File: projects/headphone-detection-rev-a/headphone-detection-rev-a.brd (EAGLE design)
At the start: 22 x 23 mm, 9 parts, among them J1 T1M-5POS, U1 VCNL4010

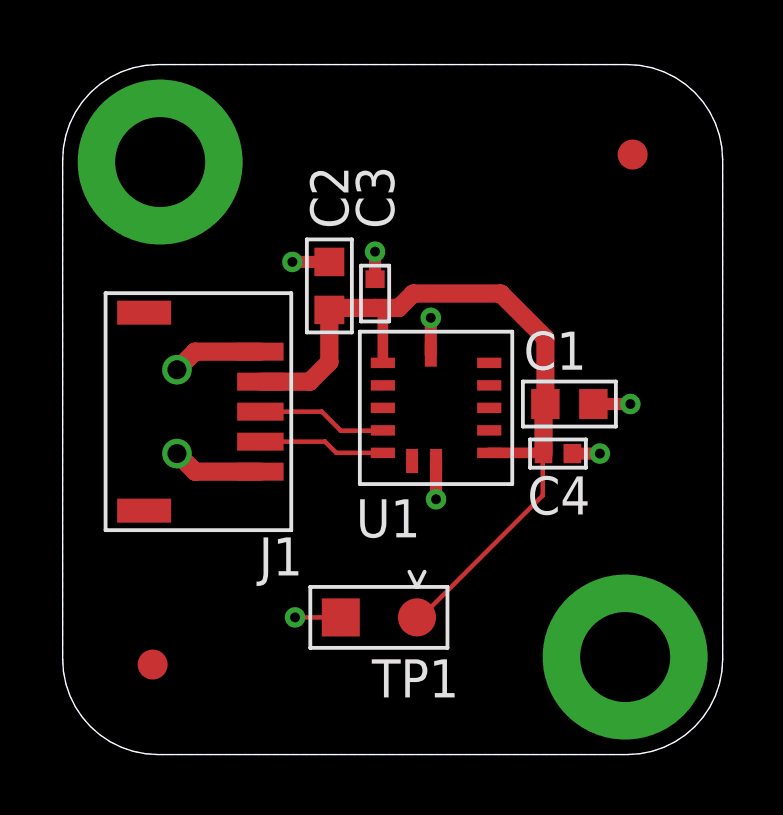
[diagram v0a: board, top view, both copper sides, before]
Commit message: Big updates to the headphone detection daughterboard.
In no particular order:

- we're now using the VL6180X (micro LIDAR, basically)
- which needs 2V8 so we have an on-board regulator
- which means we need to interface with 3V3 I2C logic so we
- added level translation FETs for each I2C line
- added test points for the two supply rails
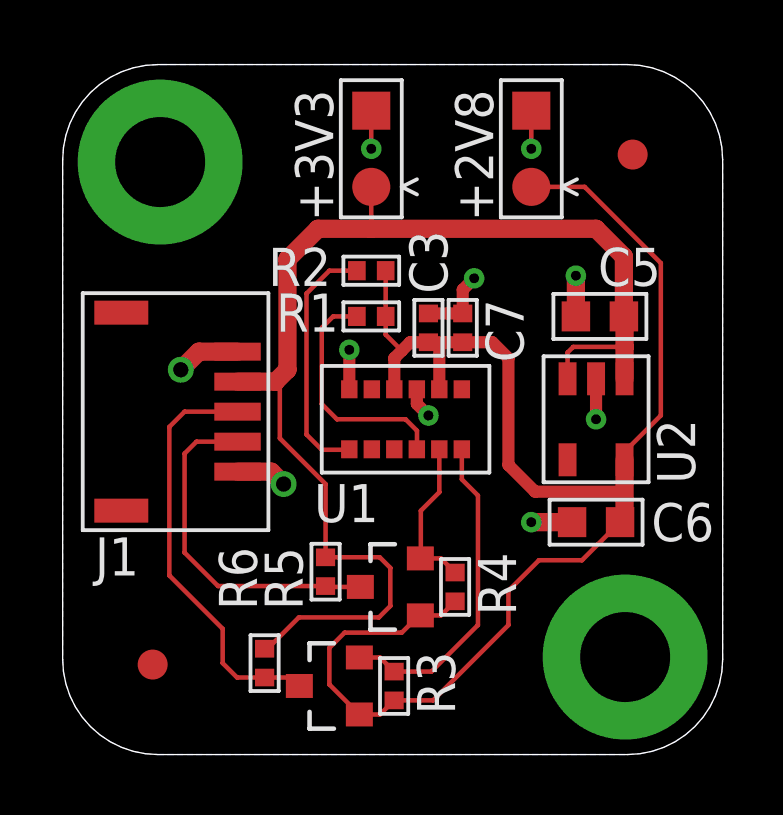
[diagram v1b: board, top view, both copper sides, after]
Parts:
- removed C1, C2: 10uF, passives:C0603
- removed C4: 1uF, passives:C0402
- added C5, C6: 10uF, passives:C0603
- added C7: 4.7uF, passives:C0402
- added R1, R2: 47K, passives:R0402
- added R3, R4, R5, R6: 10K, passives:R0402
- added TP2: TESTPOINT-WITH-GND, test:TESTPOINT-1.5-WITH-GND
- added U2: LP5907MFX-2.8, texas-instruments:R-PDSO-G5-DBV
- added U3, U4: BSS138, on-semiconductor:SOT23
- C3: value 1uF -> 100nF
- U1: value VCNL4010 -> VL6180XV0NR; device vishay:VCNL4010 -> st-microelectronics:VL6180X
- moved TP1 15.6 mm to (10.3, 20.2), turned to 90 degrees
- moved C3 2.11 mm to (12.2, 14.2)
- moved U1 1.09 mm to (11.4, 11.2), turned to 0 degrees
- moved J1 0.76 mm to (3.05, 11.4)
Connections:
- removed net N$4: J1.4, U1.SCL
- removed net N$6: J1.3, U1.SDA
- new net +2V8: C3.1, C6.1, C7.1, R1.2, R2.2, R3.2, R4.2, TP2.S, U1.10, U1.8, U2.5, U3.1, U4.1
- new net LOCAL_SCL: R4.1, U1.5, U3.2
- new net LOCAL_SDA: R3.1, U1.6, U4.2
- new net N$3: R2.1, U1.1
- new net N$5: R1.1, U1.4
- new net SCL: J1.4, R5.1, U3.3
- new net SDA: J1.3, R6.1, U4.3
- net +3V3: now also C5.1, R5.2, R6.2, U2.1, U2.3; no longer C1.1, C2.1, C3.1, C4.1, U1.IR_ANODE, U1.VDD
- net AGND: now also C5.2, C6.2, C7.2, TP2.G, U1.12, U1.9, U2.2; no longer C1.2, C2.2, C4.2, U1.GND1, U1.GND2
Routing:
- net +2V8: track 0.00 -> 52.7 mm
- net SDA: track 0.00 -> 14.0 mm
- net +3V3: track 27.3 -> 40.8 mm
- net SCL: track 0.00 -> 11.6 mm
- net LOCAL_SDA: track 0.00 -> 10.9 mm
- net N$3: track 0.00 -> 8.34 mm
- net N$5: track 0.00 -> 8.03 mm
- net LOCAL_SCL: track 0.00 -> 5.25 mm
- net N$6: track 4.35 -> 0.00 mm
- net N$4: track 4.24 -> 0.00 mm
- net AGND: track 14.4 -> 15.3 mm, vias 9 -> 10
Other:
- board text added: "+2V8"
- board text added: "+3V3"
